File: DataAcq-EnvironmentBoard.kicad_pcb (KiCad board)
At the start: 2 copper layers, 56.1 x 59 mm, 29 parts, among them J1 Airflow Breakout, J2 CAN Output, J3 CAN Input, J4 Humidity Breakout, J5 Temp Breakout, U4 Daughterboard Connector

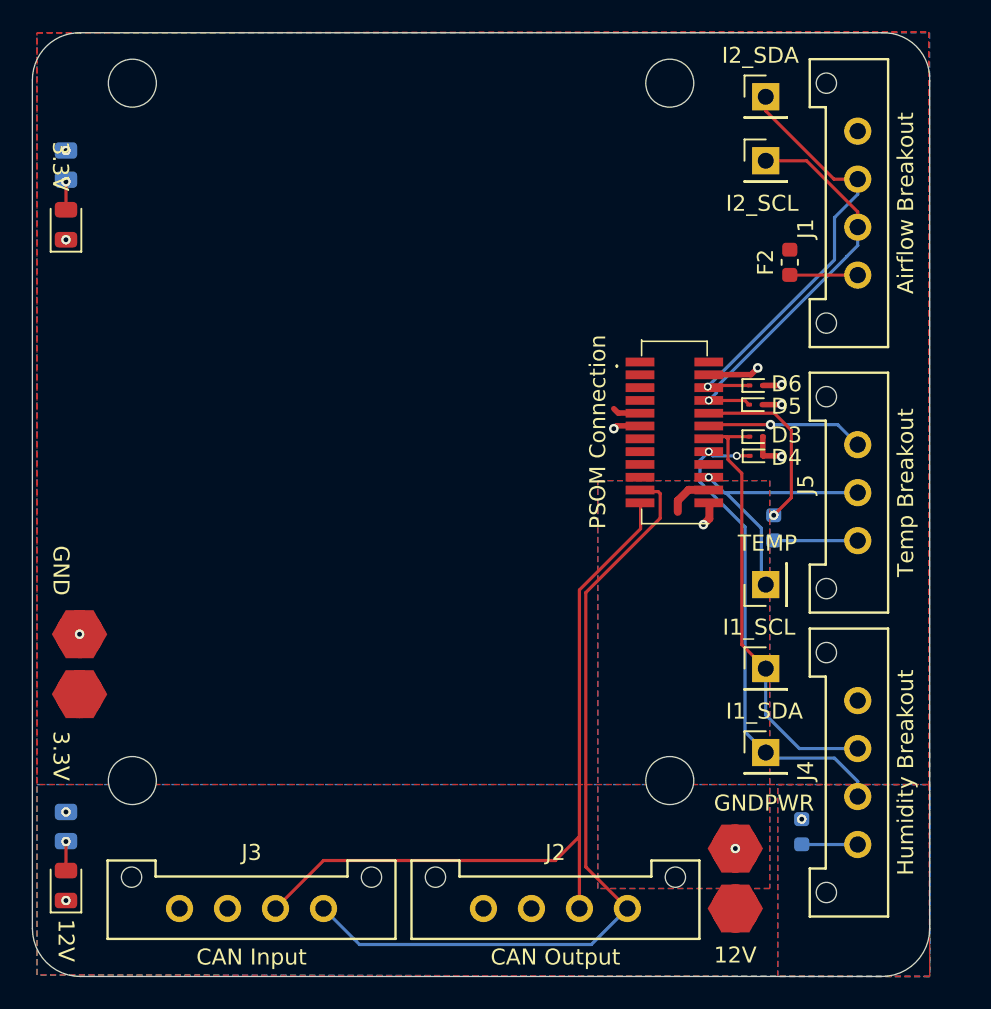
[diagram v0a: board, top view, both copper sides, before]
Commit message: modify layout for new connector
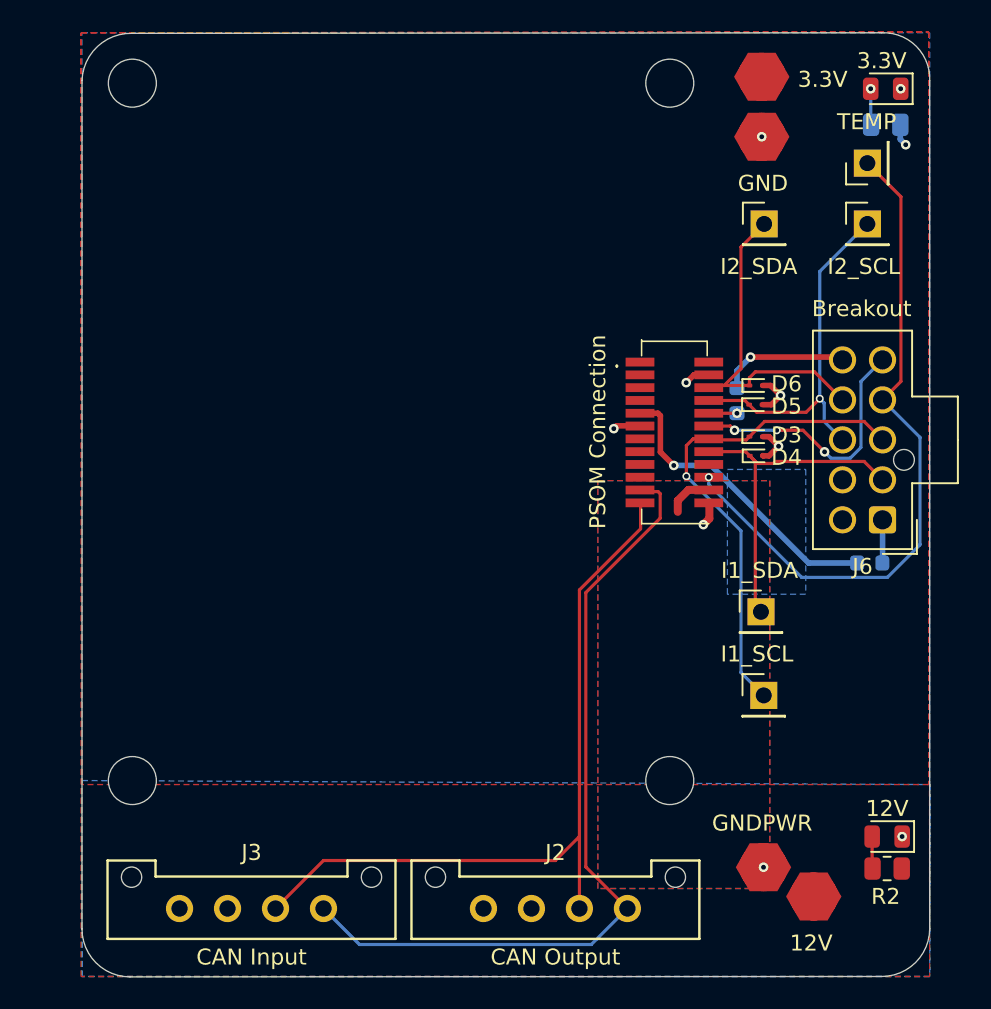
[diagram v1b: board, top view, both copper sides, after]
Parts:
- removed F3: 250mA, Fuse:Fuse_0603_1608Metric
- removed J1: Airflow Breakout, UTSVT_Connectors:Molex_MicroFit3.0_1x4xP3.00mm_PolarizingPeg_Vertical
- removed J4: Humidity Breakout, UTSVT_Connectors:Molex_MicroFit3.0_1x4xP3.00mm_PolarizingPeg_Vertical
- removed J5: Temp Breakout, UTSVT_Connectors:Molex_MicroFit3.0_1x3xP3.00mm_PolarizingPeg_Vertical
- added J6: Breakout Connector, Connector_Molex:Molex_Nano-Fit_105310-xx10_2x05_P2.50mm_Vertical, F.Cu at (192.8, 101.7)
- F2: moved to B.Cu
- R2: moved to F.Cu
- moved TP4 57.5 mm to (185.2, 74.0)
- moved TP5 52.8 mm to (185.2, 77.8)
- moved D2 52.0 mm to (193.0, 74.8), turned to 180 degrees
- moved D1 51.4 mm to (193.1, 121.5), turned to 180 degrees
- moved R2 51.4 mm to (193.1, 123.5), turned to 180 degrees
- moved R3 51.3 mm to (193.0, 77.0), turned to 180 degrees
- moved TP3 27.1 mm to (191.8, 79.4)
- moved F1 17.3 mm to (192.0, 104.4), turned to 0 degrees
- moved F2 9.26 mm to (183.7, 94.2)
- moved TP6 8.81 mm to (185.2, 107.5)
- moved TP8 7.95 mm to (185.4, 83.2)
- moved TP9 7.48 mm to (191.8, 83.2)
- moved TP1 4.96 mm to (188.5, 125.2), turned to 90 degrees
- moved TP2 2.11 mm to (185.4, 123.4)
- moved TP7 1.68 mm to (185.4, 112.7)
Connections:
- F1 pad 2: Net-(J4-Pin_1) -> /3.3-out
- F2 pad 1: +3.3V -> /VDDA-out
- F2 pad 2: Net-(J1-Pin_1) -> VDDA
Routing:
- net /PA1(ADC): track 16.6 -> 43.1 mm
- net +3.3V: track 1.79 -> 20.2 mm
- net VDDA: track 11.4 -> 1.76 mm
- net /I2C1_SDA: track 30.9 -> 21.7 mm, vias 2 -> 0
- net /VDDA-out: track 0.00 -> 8.11 mm, vias 0 -> 1
- net /I2C2_SDA: track 27.9 -> 20.9 mm, vias 1 -> 0
- net GNDA: track 9.87 -> 16.7 mm, vias 1 -> 3
- net Net-(J5-Pin_1): track 5.26 -> 0.00 mm
- net Net-(J1-Pin_1): track 4.26 -> 0.00 mm
- net Net-(J4-Pin_1): track 3.51 -> 0.00 mm
- net /I2C1_SCL: track 27.7 -> 31.0 mm, vias 0 -> 1
- net /3.3-out: track 0.00 -> 2.71 mm
- net /I2C2_SCL: track 25.4 -> 22.9 mm
- net GND: track 9.74 -> 8.60 mm, vias 7 -> 6
- net Net-(D2-A): track 1.75 -> 2.26 mm
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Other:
- board size 56.1 x 59 mm -> 53 x 59 mm
- board text added: "Breakout"
- board text removed: "Airflow Breakout"
- board text removed: "Humidity Breakout"
- board text removed: "Temp Breakout"
